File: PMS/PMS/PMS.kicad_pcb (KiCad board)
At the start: 4 copper layers, 82.5 x 57.5 mm, 32 parts, among them IC1 TMCS1107A1BQDRQ1, IC2 ADR3450ARJZ-R7, J1 XT60PW-M, J2 XT60PW-F, J3 XT60PW-M, J4 XT60PW-F, J5 XT60PW-F, J6 Conn_01x03_Male, J7 Conn_01x02_Male, U1 ADC101C027CIMK, U2 ADC101C027CIMK

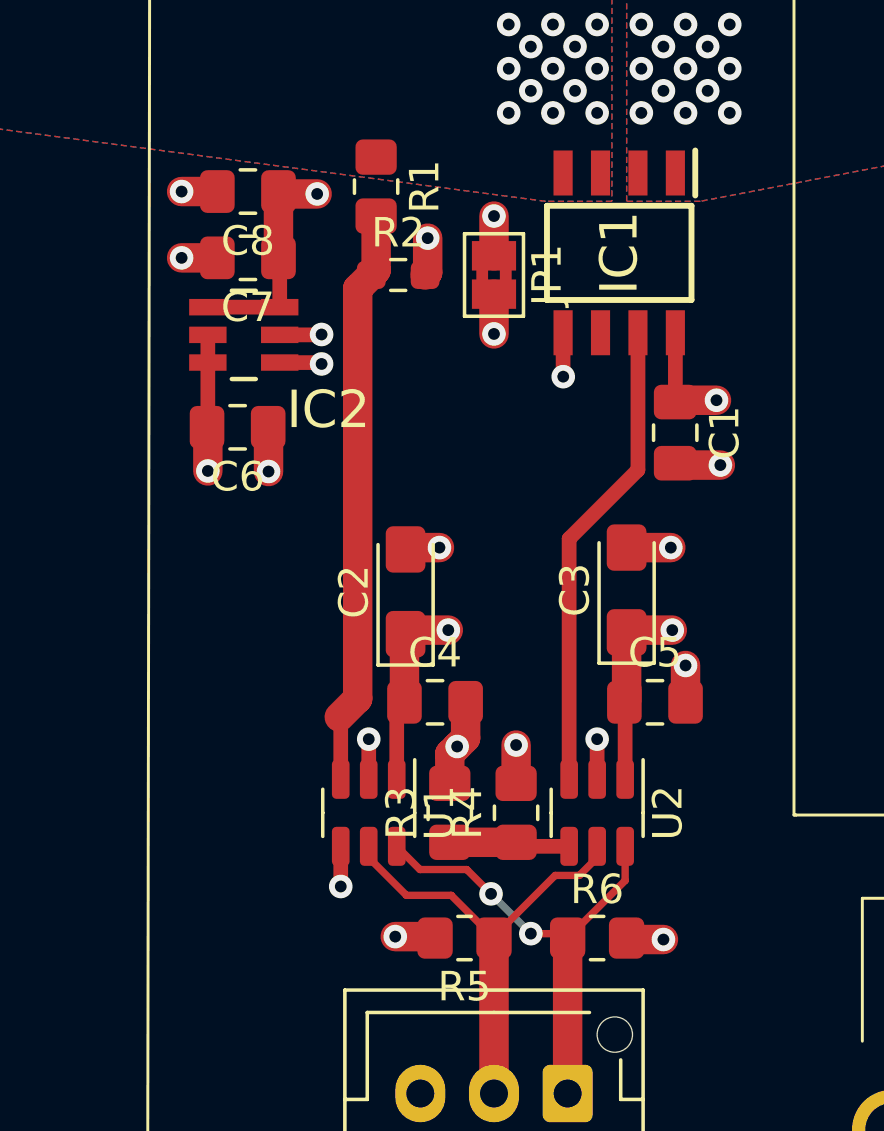
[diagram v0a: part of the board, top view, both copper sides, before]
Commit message: cleanup
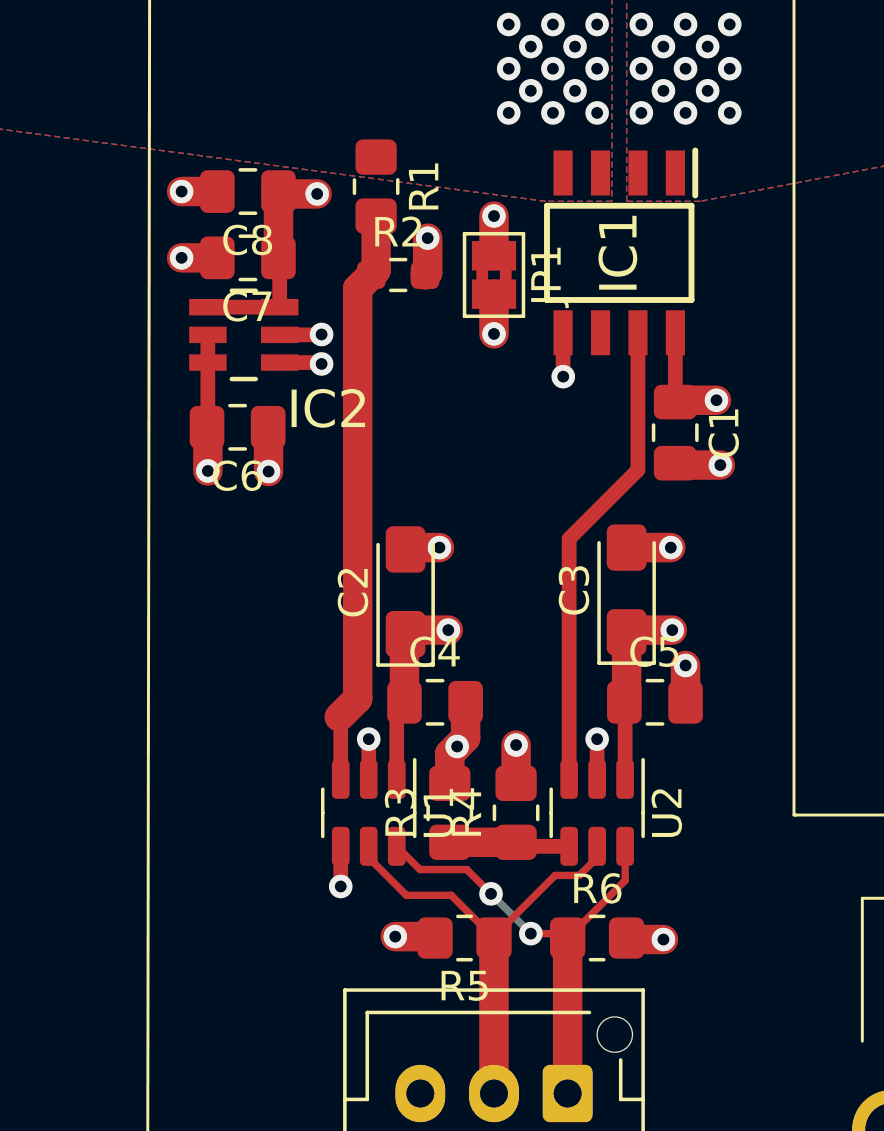
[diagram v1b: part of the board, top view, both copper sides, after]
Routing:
- net +5VA: track 25.5 -> 24.3 mm
- net SCL: track 16.1 -> 15.3 mm
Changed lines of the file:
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@@
   )
   (segment (start 106.25 86.375) (end 106.25 88.675) (width 1) (layer "F.Cu") (net 1))
-  (segment (start 98.45 89.0125) (end 98.7125 88.75) (width 0.5) (layer "F.Cu") (net 1))
-  (segment (start 107.905 78.5575) (end 107.9 78.5625) (width 0.5) (layer "F.Cu") (net 1))
   (segment (start 98.7125 88.75) (end 98.7125 86.475) (width 1) (layer "F.Cu") (net 1))
-  (segment (start 98.7125 86.475) (end 98.75 86.4375) (width 1) (layer "F.Cu") (net 1))
   (segment (start 106.2 91.3625) (end 106.2 88.775) (width 0.5) (layer "F.Cu") (net 1))
-  (segment (start 106.3 96.8) (end 106.25 96.75) (width 1) (layer "F.Cu") (net 1))
-  (segment (start 106.325 86.3) (end 106.25 86.375) (width 1) (layer "F.Cu") (net 1))
-  (segment (start 107.9625 78.5) (end 107.9 78.5625) (width 1) (layer "F.Cu") (net 1))
-  (segment (start 106.25 88.675) (end 106.175 88.75) (width 1) (layer "F.Cu") (net 1))
   (segment (start 107.905 76.211) (end 107.905 78.5575) (width 0.5) (layer "F.Cu") (net 1))
   (segment (start 98.4 96.7) (end 99.7 96.7) (width 1) (layer "F.Cu") (net 1))
   (segment (start 102.5 90.2) (end 102.5 91.5) (width 1) (layer "F.Cu") (net 1))
-  (segment (start 106.2 88.775) (end 106.175 88.75) (width 0.5) (layer "F.Cu") (net 1))
   (segment (start 92.0408 76.28195) (end 92.0408 77.22175) (width 0.5) (layer "F.Cu") (net 1))
   (segment (start 107.5 96.8) (end 106.3 96.8) (width 1) (layer "F.Cu") (net 1))
-  (segment (start 99.7 96.7) (end 99.75 96.75) (width 1) (layer "F.Cu") (net 1))
   (segment (start 100.2 86.3) (end 98.8875 86.3) (width 1) (layer "F.Cu") (net 1))
   (segment (start 98.45 91.3625) (end 98.45 89.0125) (width 0.5) (layer "F.Cu") (net 1))
   (segment (start 92.0408 77.22175) (end 92.0408 79.3592) (width 0.5) (layer "F.Cu") (net 1))
-  (segment (start 92.0408 79.44705) (end 92.0125 79.41875) (width 1) (layer "F.Cu") (net 1))
   (segment (start 107.8 86.3) (end 106.325 86.3) (width 1) (layer "F.Cu") (net 1))
   (segment (start 92.0408 80.9) (end 92.0408 79.44705) (width 1) (layer "F.Cu") (net 1))
-  (segment (start 92.0408 79.3592) (end 92.0408 79.39045) (width 0.5) (layer "F.Cu") (net 1))
   (segment (start 109.3 78.5) (end 107.9625 78.5) (width 1) (layer "F.Cu") (net 1))
-  (segment (start 98.8875 86.3) (end 98.75 86.4375) (width 1) (layer "F.Cu") (net 1))
   (via (at 107.8 86.3) (size 0.8) (drill 0.4) (layers "F.Cu" "B.Cu") (free) (net 1))
   (via (at 100.2 86.3) (size 0.8) (drill 0.4) (layers "F.Cu" "B.Cu") (free) (net 1))
@@
   (segment (start 94.4792 75.34215) (end 94.4792 73.71045) (width 0.5) (layer "F.Cu") (net 6))
   (segment (start 95.75 71.5) (end 94.51875 71.5) (width 1) (layer "F.Cu") (net 6))
-  (segment (start 94.51875 71.5) (end 94.4375 71.41875) (width 1) (layer "F.Cu") (net 6))
   (segment (start 92.0408 75.34215) (end 94.4792 75.34215) (width 0.5) (layer "F.Cu") (net 6))
   (via (at 95.75 71.5) (size 0.8) (drill 0.4) (layers "F.Cu" "B.Cu") (free) (net 6))
@@
   (segment (start 106.2 93.6375) (end 106.2 94.8) (width 0.25) (layer "F.Cu") (net 10))
   (segment (start 99.23702 94.42452) (end 98.45 93.6375) (width 0.25) (layer "F.Cu") (net 10))
-  (segment (start 104.1 96.6) (end 104.25 96.75) (width 0.25) (layer "F.Cu") (net 10))
   (segment (start 103 96.6) (end 104.1 96.6) (width 0.25) (layer "F.Cu") (net 10))
   (via (at 101.65 95.25) (size 0.8) (drill 0.4) (layers "F.Cu" "B.Cu") (net 10))
@@
   (segment (start 100.3 95.3) (end 98.778928 95.3) (width 0.25) (layer "F.Cu") (net 11))
   (segment (start 101.75 96.75) (end 100.3 95.3) (width 0.25) (layer "F.Cu") (net 11))
-  (segment (start 105.25 93.6375) (end 105.25 94.021072) (width 0.25) (layer "F.Cu") (net 11))
   (segment (start 105.25 94.021072) (end 104.646552 94.62452) (width 0.25) (layer "F.Cu") (net 11))
   (segment (start 101.75 102.025) (end 101.75 96.75) (width 1) (layer "F.Cu") (net 11))
   (segment (start 98.778928 95.3) (end 97.5 94.021072) (width 0.25) (layer "F.Cu") (net 11))
   (segment (start 103.82548 94.62452) (end 101.75 96.7) (width 0.25) (layer "F.Cu") (net 11))
-  (segment (start 97.5 94.021072) (end 97.5 93.6375) (width 0.25) (layer "F.Cu") (net 11))
-  (segment (start 101.75 96.7) (end 101.75 96.75) (width 0.25) (layer "F.Cu") (net 11))
   (segment (start 104.646552 94.62452) (end 103.82548 94.62452) (width 0.25) (layer "F.Cu") (net 11))
   (segment (start 97.12548 88.62452) (end 97.12548 74.71202) (width 1) (layer "F.Cu") (net 13))
@@
   (segment (start 97.75 74.0875) (end 97.75 72.25) (width 1) (layer "F.Cu") (net 13))
   (segment (start 104.3 93.6375) (end 102.6375 93.6375) (width 0.5) (layer "F.Cu") (net 14))
-  (segment (start 102.6375 93.6375) (end 102.5 93.5) (width 0.5) (layer "F.Cu") (net 14))
   (segment (start 100.25 93.5) (end 102.5 93.5) (width 1) (layer "F.Cu") (net 14))
   (segment (start 100.25 90.5) (end 100.5 90.25) (width 1) (layer "F.Cu") (net 15))
@@
   (segment (start 101.75 74.9) (end 101.75 76.25) (width 1) (layer "F.Cu") (net 15))
   (segment (start 94.4792 77.22175) (end 95.853 77.22175) (width 0.5) (layer "F.Cu") (net 15))
-  (segment (start 107.9625 80.7) (end 107.9 80.6375) (width 1) (layer "F.Cu") (net 15))
   (segment (start 108.25 88.75) (end 108.25 87.5) (width 1) (layer "F.Cu") (net 15))
   (segment (start 100.7875 88.75) (end 100.7875 89.9625) (width 1) (layer "F.Cu") (net 15))
@@
   (segment (start 104.095 77.695) (end 104.1 77.7) (width 0.5) (layer "F.Cu") (net 15))
   (segment (start 97.5 91.3625) (end 97.5 90) (width 0.5) (layer "F.Cu") (net 15))
-  (segment (start 98.8125 83.5) (end 98.75 83.5625) (width 1) (layer "F.Cu") (net 15))
   (segment (start 107.75 83.5) (end 106.25 83.5) (width 1) (layer "F.Cu") (net 15))
   (segment (start 104.095 76.211) (end 104.095 77.695) (width 0.5) (layer "F.Cu") (net 15))
